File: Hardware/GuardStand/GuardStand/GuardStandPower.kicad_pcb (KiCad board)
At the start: 2 copper layers, 91.4 x 90.2 mm, 48 parts, among them J1 BATT, J2 DIS, J3 12V, J4 12V, J5 12V, J6 12V, J7 15-18VAC, Q1 BC549, Q2 BC549, U1 LM317_TO-220, U2 LM317_TO-220

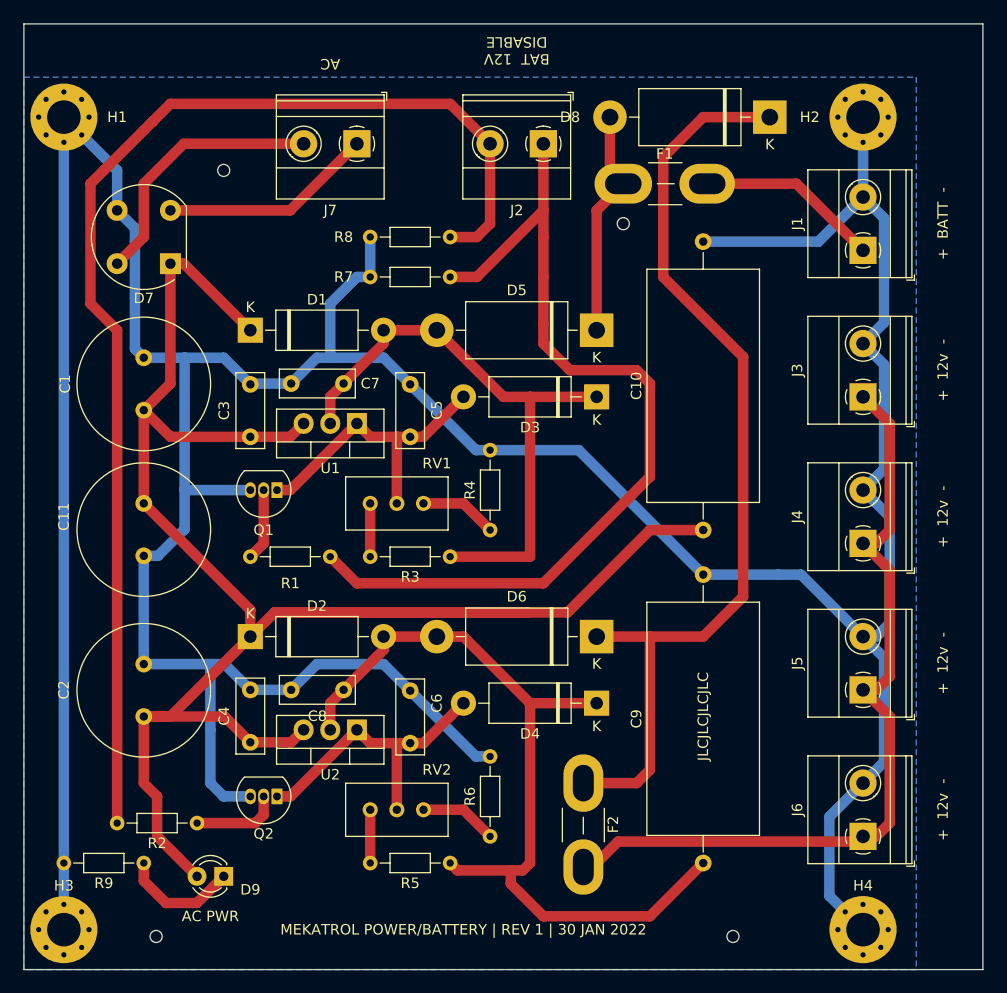
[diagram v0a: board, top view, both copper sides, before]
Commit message: Design updates
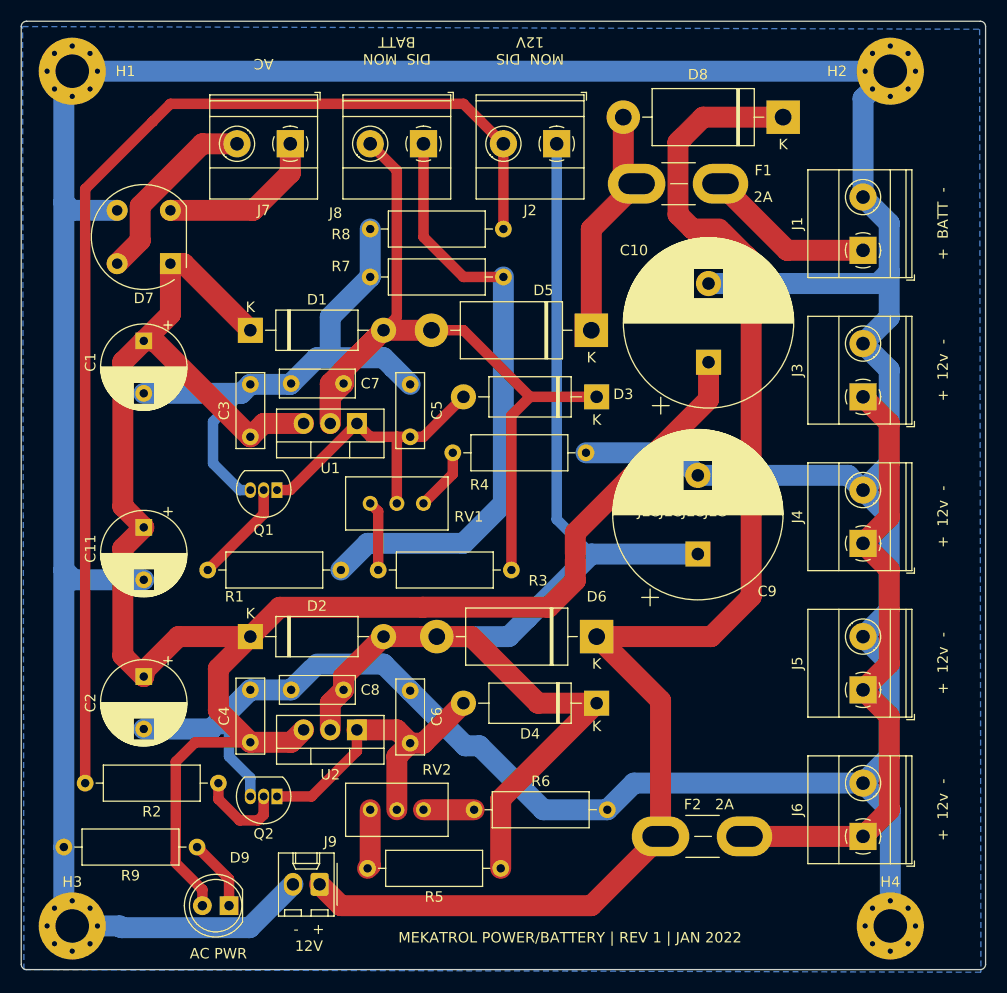
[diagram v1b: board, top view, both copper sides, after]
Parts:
- added J8: DIS, TerminalBlock_Phoenix:TerminalBlock_Phoenix_MKDS-1,5-2-5.08_1x02_P5.08mm_Horizontal, F.Cu at (110.5, 58.4)
- added J9: 12v, Connector_Molex:Molex_KK-254_AE-6410-02A_1x02_P2.54mm_Vertical, F.Cu at (100.6, 129.0)
- C1, C11, C2: footprint Capacitor_THT:C_Radial_D12.5mm_H25.0mm_P5.00mm -> Capacitor_THT:CP_Radial_D8.0mm_P5.00mm
- C10, C9: footprint Capacitor_THT:C_Axial_L22.0mm_D10.5mm_P27.50mm_Horizontal -> Capacitor_THT:CP_Radial_D16.0mm_P7.50mm
- D9: footprint LED_THT:LED_D3.0mm -> LED_THT:LED_D5.0mm
- R1, R2, R3, R4, R5, R6, R7, R8, R9: footprint Resistor_THT:R_Axial_DIN0204_L3.6mm_D1.6mm_P7.62mm_Horizontal -> Resistor_THT:R_Axial_DIN0309_L9.0mm_D3.2mm_P12.70mm_Horizontal
- moved C9 29.5 mm to (136.7, 97.5)
- moved C10 16.0 mm to (137.7, 79.2)
- moved F2 8.95 mm to (133.1, 124.5), turned to 0 degrees
- moved R4 8.18 mm to (113.3, 87.9), turned to 0 degrees
- moved C1 6.60 mm to (83.8, 77.2), turned to 270 degrees
- moved J7 6.35 mm to (97.8, 58.4)
- moved R3 5.98 mm to (118.9, 99.1)
- moved R9 5.30 mm to (88.9, 125.5)
- moved H2 5.09 mm to (155.0, 51.5)
- moved R5 4.85 mm to (117.9, 127.5)
- moved H1 4.45 mm to (77.0, 51.5)
- moved R2 4.32 mm to (90.9, 119.4)
- moved R1 4.26 mm to (89.9, 99.1)
- moved C2 3.81 mm to (83.8, 109.2), turned to 270 degrees
- moved R6 2.96 mm to (115.3, 121.9), turned to 0 degrees
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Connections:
- net +BATT renamed BATT_SUP
- C8 pad 1: +12V -> 12V_SUP
- C9 pad 1: +12V -> 12V_SUP
- D2 pad 2: +12V -> 12V_SUP
- D4 pad 1: +12V -> 12V_SUP
- D6 pad 2: +12V -> 12V_SUP
- J2 pad 1: BATT_DIS -> 12V_SUP
- R5 pad 1: +12V -> 12V_SUP
- U2 pad 2: +12V -> 12V_SUP
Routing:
- net 12V_SUP: track 0.00 -> 132.8 mm
- net GND: track 396.4 -> 496.0 mm
- net +12V: track 80.4 -> 0.00 mm
- net Net-(D6-Pad1): track 91.9 -> 140.0 mm
- net BATT_DIS: track 86.9 -> 57.8 mm
- net BATT_SUP: track 56.8 -> 80.5 mm
- net Net-(F2-Pad2): track 78.3 -> 59.4 mm
- net Net-(D7-Pad4): track 25.5 -> 18.1 mm
- net 12V_DIS: track 116.8 -> 109.6 mm
- net Net-(D7-Pad2): track 20.4 -> 15.7 mm
- net Net-(D9-Pad1): track 11.2 -> 6.85 mm
- net Net-(Q1-Pad2): track 6.88 -> 9.83 mm
- net Net-(R6-Pad1): track 7.40 -> 4.83 mm
- net Net-(C6-Pad1): track 28.9 -> 30.6 mm
- net Net-(R3-Pad2): track 5.08 -> 6.67 mm
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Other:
- board size 91.4 x 90.2 mm -> 91.9 x 90.4 mm
- board text added: "- + 12V"
- board text added: "2A"
- board text added: "DIS MON BATT"
- board text added: "MEKATROL POWER/BATTERY | REV 1 | JAN 2022"
- board text added: "MON DIS 12V"
- board text removed: "BAT 12V DISABLE"
- board text removed: "MEKATROL POWER/BATTERY | REV 1 | 30 JAN 2022"
